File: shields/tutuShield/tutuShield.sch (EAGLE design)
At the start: 6 parts, among them IC1 IC_MSGEQ7-SOIC8

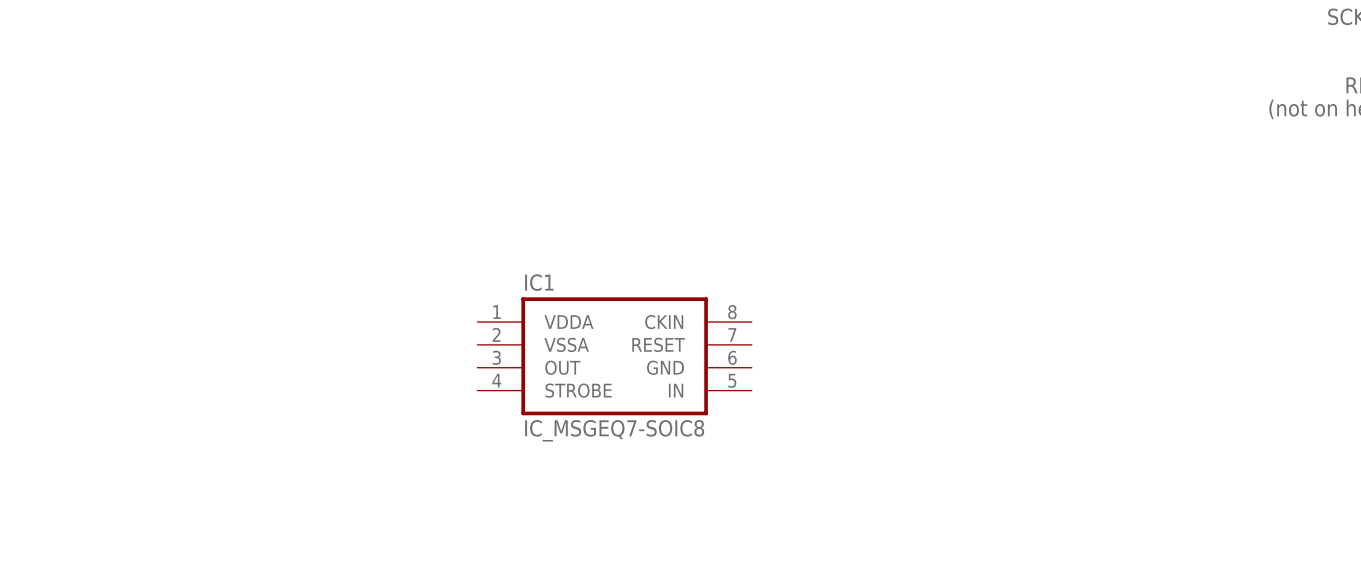
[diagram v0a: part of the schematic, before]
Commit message: didn't save last time :\
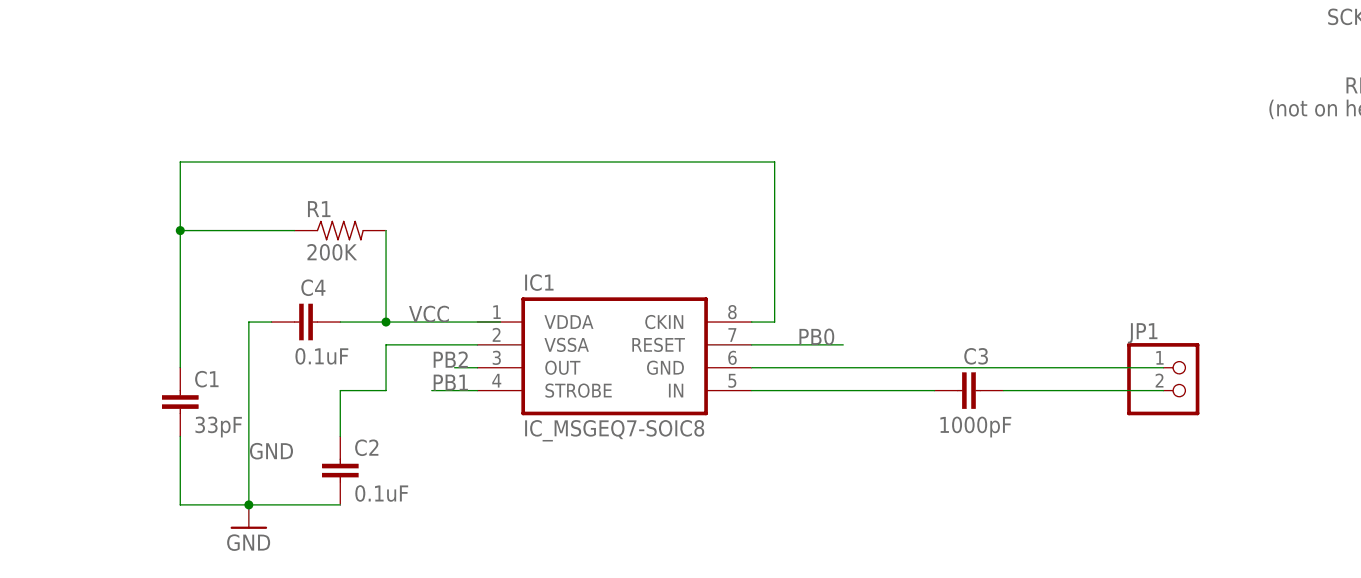
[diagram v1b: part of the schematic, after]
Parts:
- added C1: 33pF, ATtami:CAP0805
- added C2, C4: 0.1uF, ATtami:CAP0805
- added C3: 1000pF, ATtami:CAP0805
- added JP1: (no value), ATtami:HEADER-1X2ROUND
- added R1: 200K, ATtami:RESISTOR0805-RES
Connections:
- new net CKIN: C1.1, IC1.CKIN, R1.1
- new net IN: C3.1, IC1.IN
- new net N$1: C3.2, JP1.2
- new net N$4: IC1.GND, JP1.1
- new net N$5: C2.1, IC1.VSSA
- net GND: now also C1.2, C2.2, C4.1
- net PB0: now also IC1.RESET
- net PB1: now also IC1.STROBE
- net PB2: now also IC1.OUT
- net VCC: now also C4.2, R1.2
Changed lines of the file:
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@@
 <?xml version="1.0" encoding="utf-8"?>
 <!DOCTYPE eagle SYSTEM "eagle.dtd">
-<eagle version="7.1.0">
+<eagle version="7.2.0">
 <drawing>
 <settings>
@@
 <part name="GND5" library="SparkFun" deviceset="GND" device=""/>
 <part name="IC1" library="ATtami" deviceset="IC_MSGEQ7" device="-SOIC8"/>
+<part name="C1" library="ATtami" deviceset="CAP" device="0805" value="33pF"/>
+<part name="C2" library="ATtami" deviceset="CAP" device="0805" value="0.1uF"/>
+<part name="C3" library="ATtami" deviceset="CAP" device="0805" value="1000pF"/>
+<part name="C4" library="ATtami" deviceset="CAP" device="0805" value="0.1uF"/>
+<part name="GND2" library="SparkFun" deviceset="GND" device=""/>
+<part name="JP1" library="ATtami" deviceset="HEADER-1X2" device="ROUND"/>
+<part name="R1" library="ATtami" deviceset="RESISTOR" device="0805-RES" value="200K"/>
 </parts>
 <sheets>
@@
 <instance part="GND5" gate="1" x="218.44" y="134.62" rot="R180"/>
 <instance part="IC1" gate="IC" x="116.84" y="83.82"/>
+<instance part="C1" gate="G$1" x="68.58" y="78.74"/>
+<instance part="C2" gate="G$1" x="86.36" y="71.12"/>
+<instance part="C3" gate="G$1" x="157.48" y="81.28" smashed="yes" rot="R90">
+<attribute name="NAME" x="158.496" y="85.979" size="1.778" layer="95" rot="R180"/>
+<attribute name="VALUE" x="161.036" y="78.359" size="1.778" layer="96" rot="R180"/>
+</instance>
+<instance part="C4" gate="G$1" x="83.82" y="88.9" smashed="yes" rot="R90">
+<attribute name="NAME" x="84.836" y="93.599" size="1.778" layer="95" rot="R180"/>
+<attribute name="VALUE" x="87.376" y="85.979" size="1.778" layer="96" rot="R180"/>
+</instance>
+<instance part="GND2" gate="1" x="76.2" y="66.04"/>
+<instance part="JP1" gate="G$1" x="180.34" y="81.28"/>
+<instance part="R1" gate="G$1" x="86.36" y="99.06"/>
 </instances>
 <busses>
@@
 <pinref part="GND5" gate="1" pin="GND"/>
 </segment>
+<segment>
+<pinref part="C4" gate="G$1" pin="1"/>
+<pinref part="GND2" gate="1" pin="GND"/>
+<wire x1="78.74" y1="88.9" x2="76.2" y2="88.9" width="0.1524" layer="91"/>
+<wire x1="76.2" y1="88.9" x2="76.2" y2="68.58" width="0.1524" layer="91"/>
+<label x="76.2" y="73.66" size="1.778" layer="95"/>
+<pinref part="C2" gate="G$1" pin="2"/>
+<wire x1="86.36" y1="68.58" x2="76.2" y2="68.58" width="0.1524" layer="91"/>
+<junction x="76.2" y="68.58"/>
+<pinref part="C1" gate="G$1" pin="2"/>
+<wire x1="68.58" y1="76.2" x2="68.58" y2="68.58" width="0.1524" layer="91"/>
+<wire x1="68.58" y1="68.58" x2="76.2" y2="68.58" width="0.1524" layer="91"/>
+</segment>
 </net>
 <net name="VCC" class="0">
@@
 <label x="86.868" y="145.288" size="1.778" layer="95"/>
 </segment>
+<segment>
+<pinref part="C4" gate="G$1" pin="2"/>
+<wire x1="104.14" y1="88.9" x2="91.44" y2="88.9" width="0.1524" layer="91"/>
+<label x="93.98" y="88.9" size="1.778" layer="95"/>
+<pinref part="R1" gate="G$1" pin="2"/>
+<wire x1="91.44" y1="88.9" x2="86.36" y2="88.9" width="0.1524" layer="91"/>
+<wire x1="91.44" y1="99.06" x2="91.44" y2="88.9" width="0.1524" layer="91"/>
+<junction x="91.44" y="88.9"/>
+</segment>
 </net>
 <net name="N$3" class="0">
@@
 <label x="218.44" y="127" size="1.778" layer="95"/>
 </segment>
+<segment>
+<pinref part="IC1" gate="IC" pin="RESET"/>
+<wire x1="132.08" y1="86.36" x2="142.24" y2="86.36" width="0.1524" layer="91"/>
+<label x="137.16" y="86.36" size="1.778" layer="95"/>
+</segment>
 </net>
 <net name="PB1" class="0">
@@
 <label x="218.44" y="124.46" size="1.778" layer="95"/>
 </segment>
+<segment>
+<pinref part="IC1" gate="IC" pin="STROBE"/>
+<wire x1="101.6" y1="81.28" x2="96.52" y2="81.28" width="0.1524" layer="91"/>
+<label x="96.52" y="81.28" size="1.778" layer="95"/>
+</segment>
 </net>
 <net name="PB2" class="0">
@@
 <label x="218.44" y="121.92" size="1.778" layer="95"/>
 </segment>
+<segment>
+<pinref part="IC1" gate="IC" pin="OUT"/>
+<wire x1="101.6" y1="83.82" x2="99.06" y2="83.82" width="0.1524" layer="91"/>
+<label x="96.52" y="83.82" size="1.778" layer="95"/>
+</segment>
 </net>
 <net name="PB3" class="0">
@@
 </segment>
 </net>
+<net name="IN" class="0">
+<segment>
+<pinref part="IC1" gate="IC" pin="IN"/>
+<pinref part="C3" gate="G$1" pin="1"/>
+<wire x1="132.08" y1="81.28" x2="152.4" y2="81.28" width="0.1524" layer="91"/>
+</segment>
+</net>
+<net name="N$1" class="0">
+<segment>
+<pinref part="C3" gate="G$1" pin="2"/>
+<pinref part="JP1" gate="G$1" pin="2"/>
+<wire x1="160.02" y1="81.28" x2="177.8" y2="81.28" width="0.1524" layer="91"/>
+</segment>
+</net>
+<net name="N$4" class="0">
+<segment>
+<pinref part="IC1" gate="IC" pin="GND"/>
+<pinref part="JP1" gate="G$1" pin="1"/>
+<wire x1="132.08" y1="83.82" x2="177.8" y2="83.82" width="0.1524" layer="91"/>
+</segment>
+</net>
+<net name="N$5" class="0">
+<segment>
+<pinref part="C2" gate="G$1" pin="1"/>
+<wire x1="86.36" y1="76.2" x2="86.36" y2="81.28" width="0.1524" layer="91"/>
+<wire x1="86.36" y1="81.28" x2="91.44" y2="81.28" width="0.1524" layer="91"/>
+<wire x1="91.44" y1="81.28" x2="91.44" y2="86.36" width="0.1524" layer="91"/>
+<pinref part="IC1" gate="IC" pin="VSSA"/>
+<wire x1="91.44" y1="86.36" x2="101.6" y2="86.36" width="0.1524" layer="91"/>
+</segment>
+</net>
+<net name="CKIN" class="0">
+<segment>
+<pinref part="IC1" gate="IC" pin="CKIN"/>
+<wire x1="132.08" y1="88.9" x2="134.62" y2="88.9" width="0.1524" layer="91"/>
+<wire x1="134.62" y1="88.9" x2="134.62" y2="106.68" width="0.1524" layer="91"/>
+<pinref part="C1" gate="G$1" pin="1"/>
+<wire x1="134.62" y1="106.68" x2="68.58" y2="106.68" width="0.1524" layer="91"/>
+<wire x1="68.58" y1="106.68" x2="68.58" y2="99.06" width="0.1524" layer="91"/>
+<pinref part="R1" gate="G$1" pin="1"/>
+<wire x1="68.58" y1="99.06" x2="68.58" y2="83.82" width="0.1524" layer="91"/>
+<wire x1="68.58" y1="99.06" x2="81.28" y2="99.06" width="0.1524" layer="91"/>
+<junction x="68.58" y="99.06"/>
+</segment>
+</net>
